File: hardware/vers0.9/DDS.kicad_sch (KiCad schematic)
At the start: 2 parts, among them U7 AD-9851

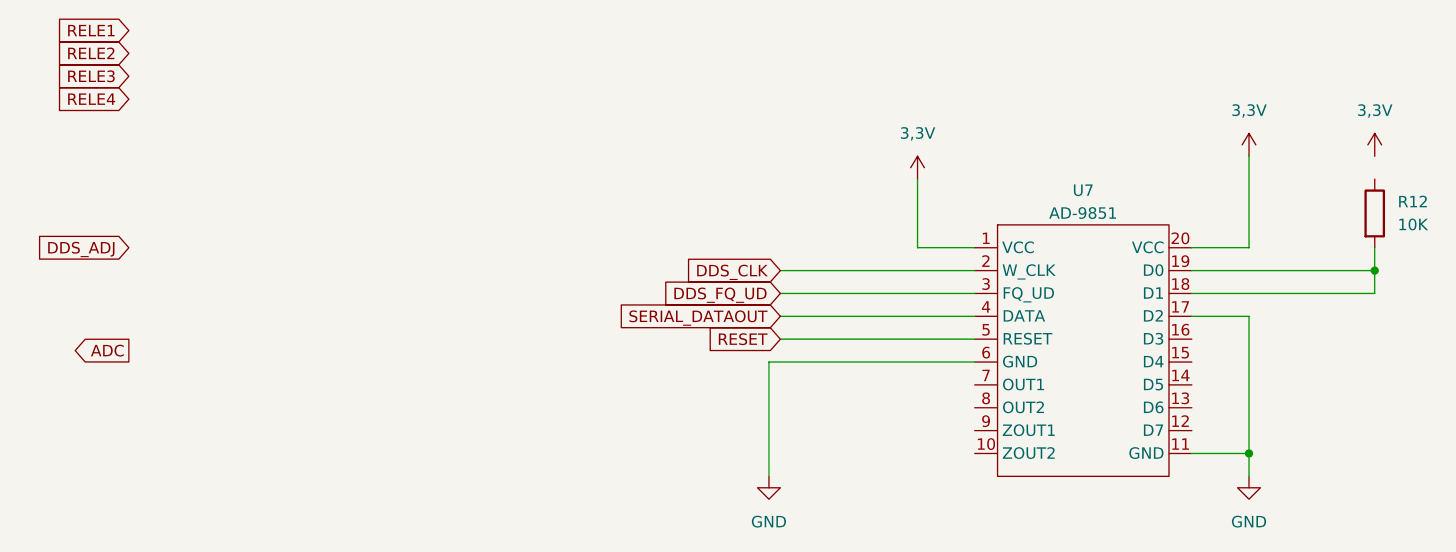
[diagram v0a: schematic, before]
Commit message: 250425-1655
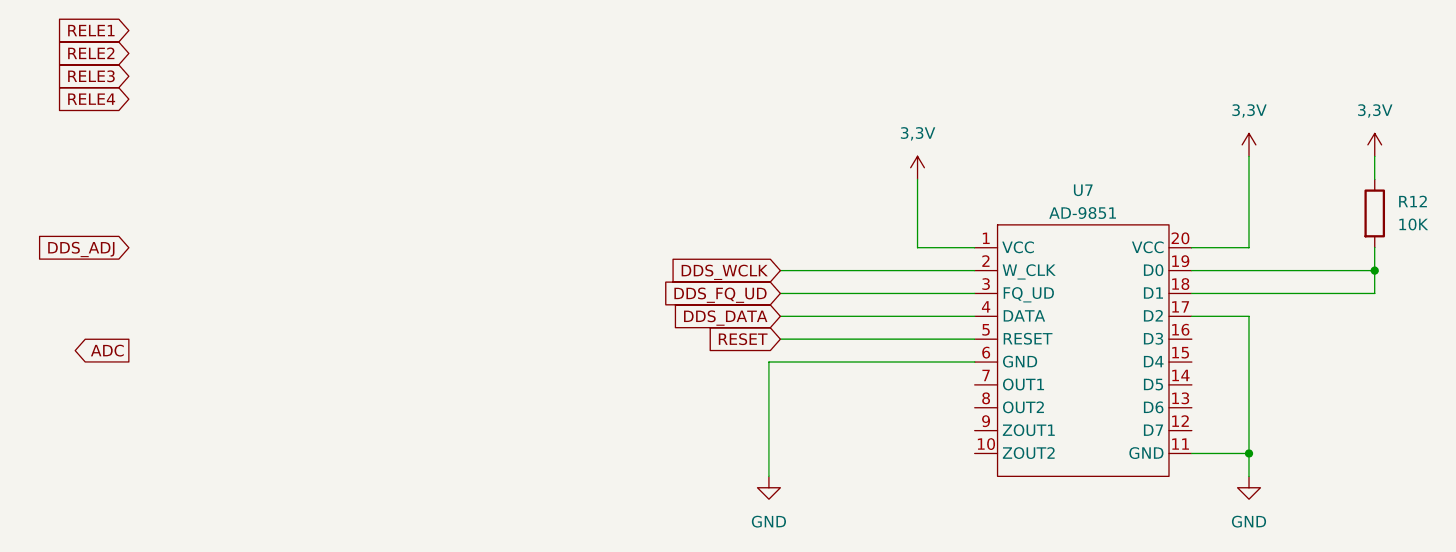
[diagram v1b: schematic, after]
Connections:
- net 3,3V: now also R12.1
- net DDS_CLK renamed DDS_WCLK
- net SERIAL_DATAOUT renamed DDS_DATA
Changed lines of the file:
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@@
+	(wire
+		(pts
+			(xy 179.07 54.61) (xy 179.07 57.15)
+		)
+		(stroke
+			(width 0)
+			(type default)
+		)
+	)
 	(wire
 		(pts
@@
 		)
 	)
-	(global_label "DDS_CLK"
+	(global_label "DDS_WCLK"
 		(shape input)
 		(at 113.03 67.31 180)
@@
 		)
 		(property "Intersheetrefs" "${INTERSHEET_REFS}"
-			(at 101.7596 67.31 0)
+			(at 100.3082 67.31 0)
 			(effects
 				(font
@@
 		)
 	)
-	(global_label "SERIAL_DATAOUT"
+	(global_label "DDS_DATA"
 		(shape input)
 		(at 113.03 72.39 180)
@@
 		)
 		(property "Intersheetrefs" "${INTERSHEET_REFS}"
-			(at 94.6838 72.39 0)
-			(effects
-				(font
+			(at 100.9129 72.39 0)
+			(effects
+				(font
